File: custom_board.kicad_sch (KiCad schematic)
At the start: 35 parts, among them IC1 TMPM46BF10FG, J1 USB_UART Conn Pins, J10 Port C, J11 Port F, J12 Port J, J2 Port G, J3 Port A, J4 Port D, J5 Port K, J6 Port L, J7 Port E, J8 Port H, J9 Port B, SW1 Boot Switch, SW2 SW_Push_Dual, Y1 HighOscillator, Y2 LowOscillator

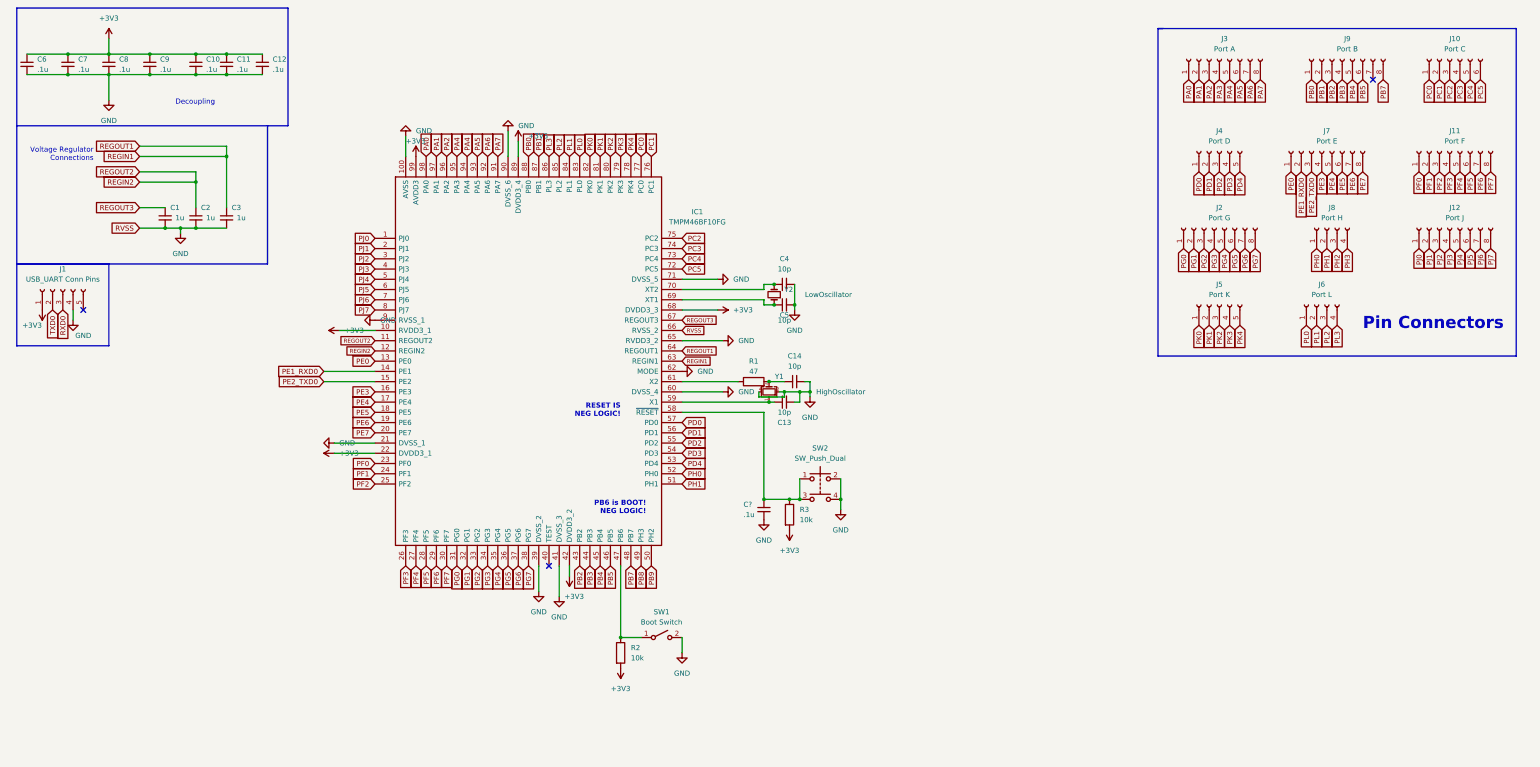
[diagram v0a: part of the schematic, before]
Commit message: idk
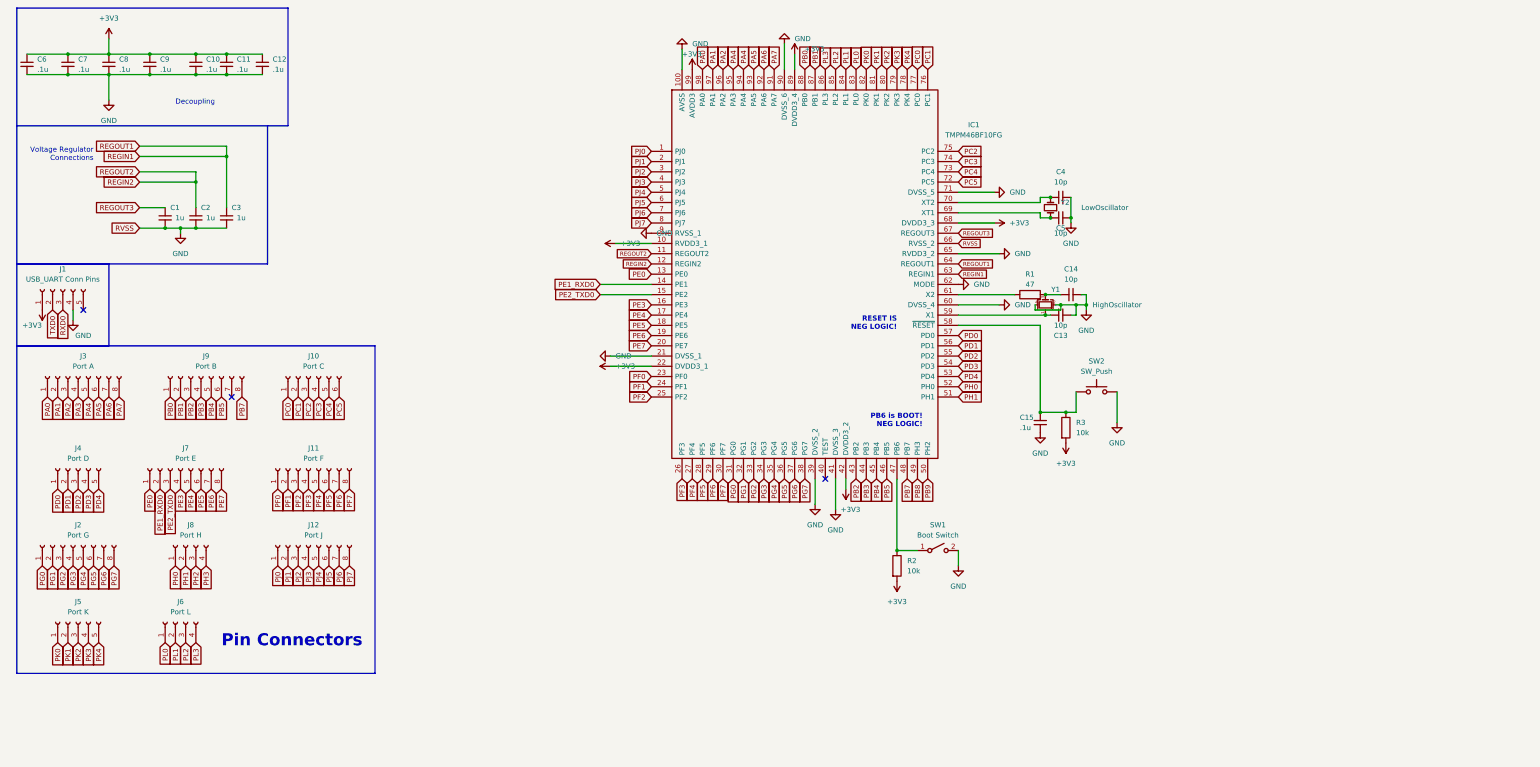
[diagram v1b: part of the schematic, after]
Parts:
- removed SW2: SW_Push_Dual, symbol Switch:SW_Push_Dual
- added SW2: SW_Push, Button_Switch_THT:Push_E-Switch_KS01Q01, symbol Switch:SW_Push
- C15: renamed from C?; footprint (none) -> Capacitor_SMD:C_0805_2012Metric
- SW1: footprint (none) -> Button_Switch_SMD:SW_DIP_SPSTx01_Slide_9.78x4.72mm_W8.61mm_P2.54mm
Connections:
- net GND: now also SW2.2
- net at C15.1, IC1.58 (~{RESET}), R3.1: now also SW2.1
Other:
- moved on the sheet: C13, C14, C15, C4, C5, IC1, J10, J11, J12, J2, J3, J4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
